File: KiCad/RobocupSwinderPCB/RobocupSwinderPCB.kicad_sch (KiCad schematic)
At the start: 29 parts, among them J1 Barrel_Jack, M1 Stepper_Motor_bipolar, M2 Stepper_Motor_bipolar, SW1 Limit_Switch, SW2 Limit_Switch, SW3 SW_SPST, U1 Teensy4.1, U3 LM7805_TO220

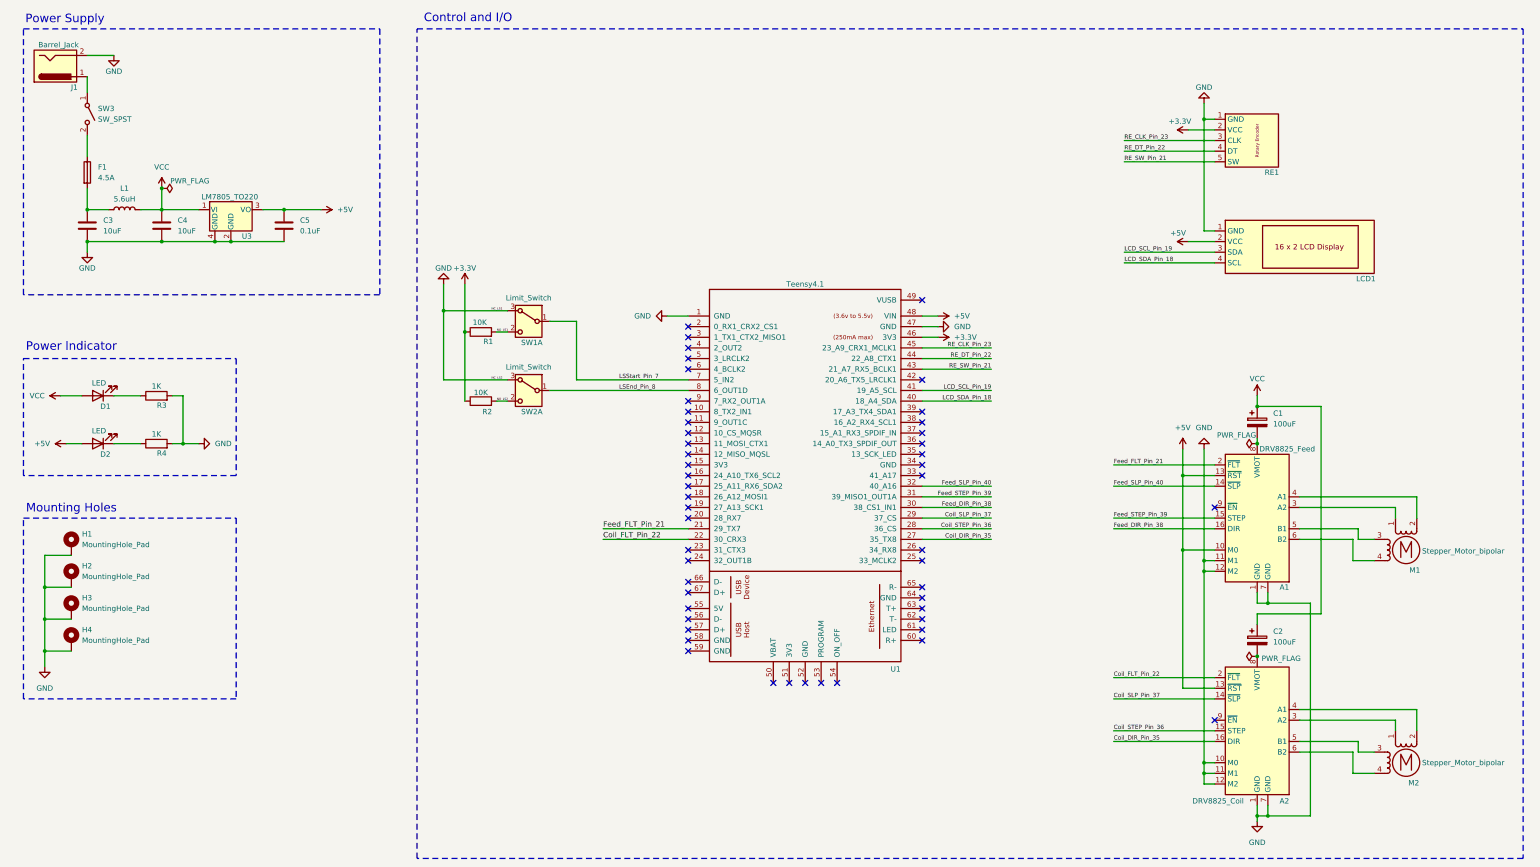
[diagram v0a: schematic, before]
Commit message: More pcb cleanup.
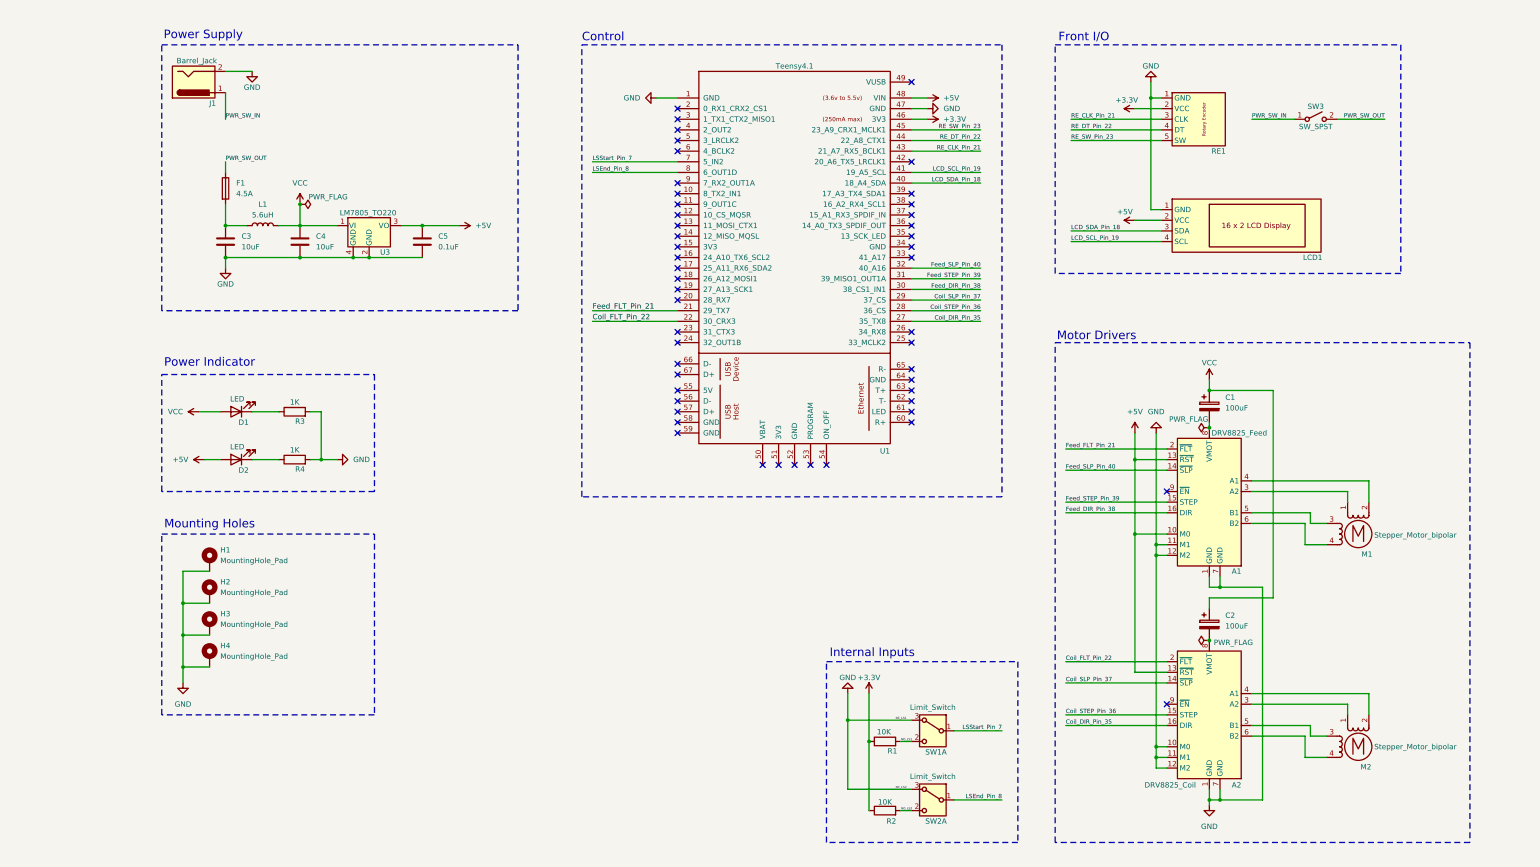
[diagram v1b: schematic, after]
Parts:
- J1: footprint Library:CUI_PJ-037A -> SwinderFootprintLibrary:CUI_PJ-037A
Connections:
- net LCD_SCL_Pin_19: now also LCD1.4 (SCL); no longer LCD1.3 (SDA)
- net LCD_SDA_Pin_18: now also LCD1.3 (SDA); no longer LCD1.4 (SCL)
- net PWR_SW_OUT: now reaches F1.1, SW3.2 (B)
- net PWR_SW_IN: now reaches J1.1, SW3.1 (A)
- net RE_CLK_Pin_23 renamed RE_CLK_Pin_21
- net RE_CLK_Pin_21: now also U1.43 (21_A7_RX5_BCLK1); no longer U1.45 (23_A9_CRX1_MCLK1)
- net RE_SW_Pin_21 renamed RE_SW_Pin_23
- net RE_SW_Pin_23: now also U1.45 (23_A9_CRX1_MCLK1); no longer U1.43 (21_A7_RX5_BCLK1)
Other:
- note added: "Control"
- note added: "Front I/O"
- note added: "Internal Inputs"
- note added: "Motor Drivers"
- note removed: "Control and I/O"
- moved on the sheet: A1, A2, C1, C2, C3, C4, C5, D1, D2, F1, H1, H2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
